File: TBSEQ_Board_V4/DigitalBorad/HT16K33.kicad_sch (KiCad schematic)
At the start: 18 parts, among them U7 HT16K33_28SOP-A_

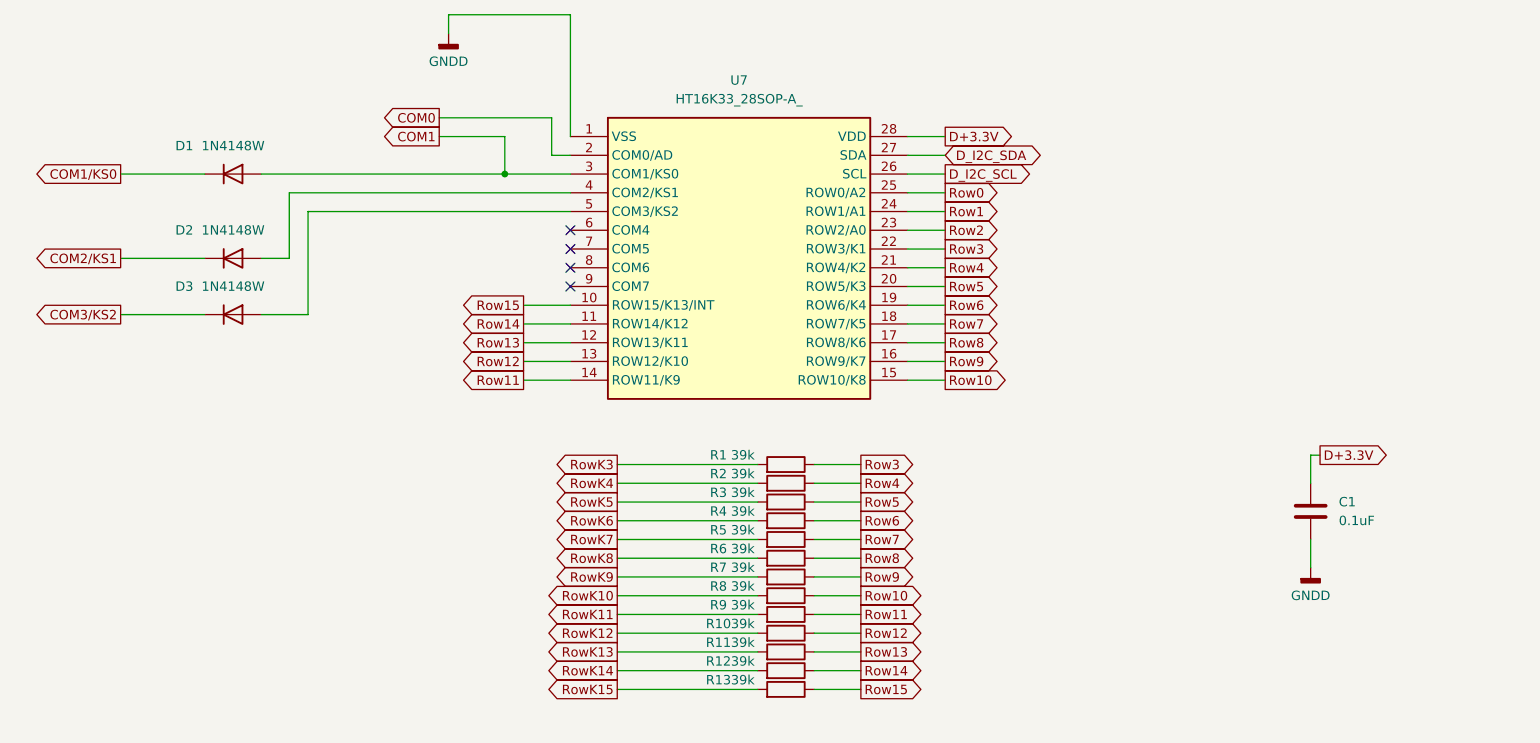
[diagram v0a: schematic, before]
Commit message: TBSEQ_BoardV4
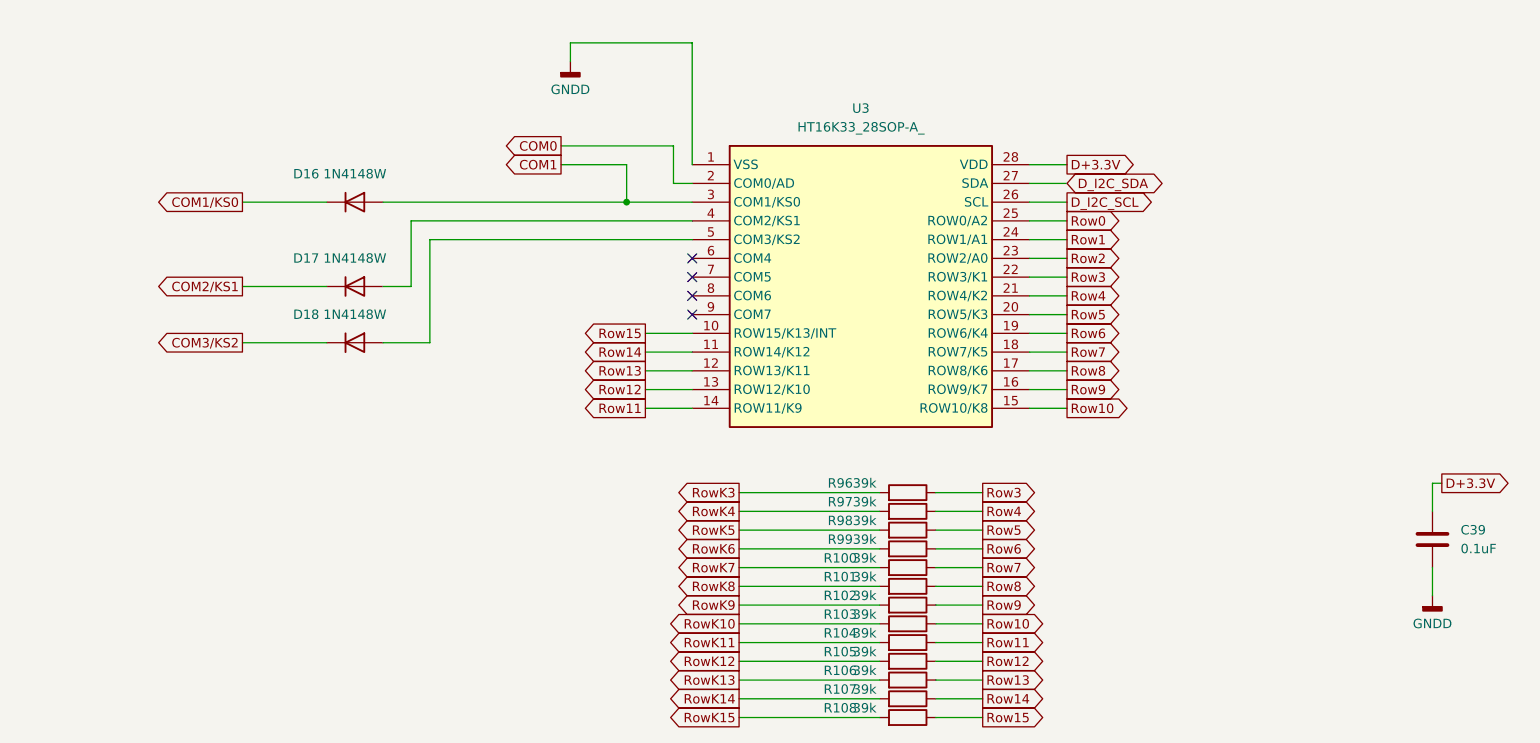
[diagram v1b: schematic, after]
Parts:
- removed C1: 0.1uF, Capacitor_SMD:C_0603_1608Metric_Pad1.08x0.95mm_HandSolder, symbol Device:C
- removed D1, D2, D3: 1N4148W, Diode_SMD:D_SOD-123, symbol Diode:1N4148W
- removed R1, R10, R11, R12, R13, R2, R3, R4, R5, R6, R7, R8, R9: 39k, Resistor_SMD:R_0603_1608Metric_Pad0.98x0.95mm_HandSolder, symbol Device:R
- added C39: 0.1uF, Capacitor_SMD:C_0805_2012Metric_Pad1.18x1.45mm_HandSolder, symbol Device:C
- added D16, D17, D18: 1N4148W, Diode_SMD:D_SOD-123, symbol Diode:1N4148W
- added R100, R101, R102, R103, R104, R105, R106, R107, R108, R96, R97, R98, R99: 39k, Resistor_SMD:R_0805_2012Metric_Pad1.20x1.40mm_HandSolder, symbol Device:R
- U3: renamed from U7; footprint SOIC127P1031X264-28N -> SamacSys_parts:SOIC127P1031X264-28N
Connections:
- net COM1: now also D16.2 (A)
- net COM1/KS0: now also D16.1 (K)
- net COM2/KS1: now also D17.1 (K)
- net COM3/KS2: now also D18.1 (K)
- net D+3.3V: now also C39.1
- net GNDD: now also C39.2
- net Row10: now also R103.1
- net Row11: now also R104.1
- net Row12: now also R105.1
- net Row13: now also R106.1
- net Row14: now also R107.1
- net Row15: now also R108.1
- net Row3: now also R96.1
- net Row4: now also R97.1
- net Row5: now also R98.1
- net Row6: now also R99.1
- net Row7: now also R100.1
- net Row8: now also R101.1
- net Row9: now also R102.1
- net RowK10: now also R103.2
- net RowK11: now also R104.2
- net RowK12: now also R105.2
- net RowK13: now also R106.2
- net RowK14: now also R107.2
- net RowK15: now also R108.2
- net RowK3: now also R96.2
- net RowK4: now also R97.2
- net RowK5: now also R98.2
- net RowK6: now also R99.2
- net RowK7: now also R100.2
- net RowK8: now also R101.2
- net RowK9: now also R102.2
- net at U3.4 (COM2/KS1): now also D17.2 (A)
- net at U3.5 (COM3/KS2): now also D18.2 (A)
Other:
- moved on the sheet: U3
